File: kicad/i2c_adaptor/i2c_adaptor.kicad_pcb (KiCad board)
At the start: 2 copper layers, 15 parts, among them J1 Conn_01x02, J2 Conn_01x05, J4 Conn_01x14, J5 Conn_01x02, J6 Conn_01x14, Q1 Fairchild BS170, SW1 SW_SPDT, U1 pic16f1825

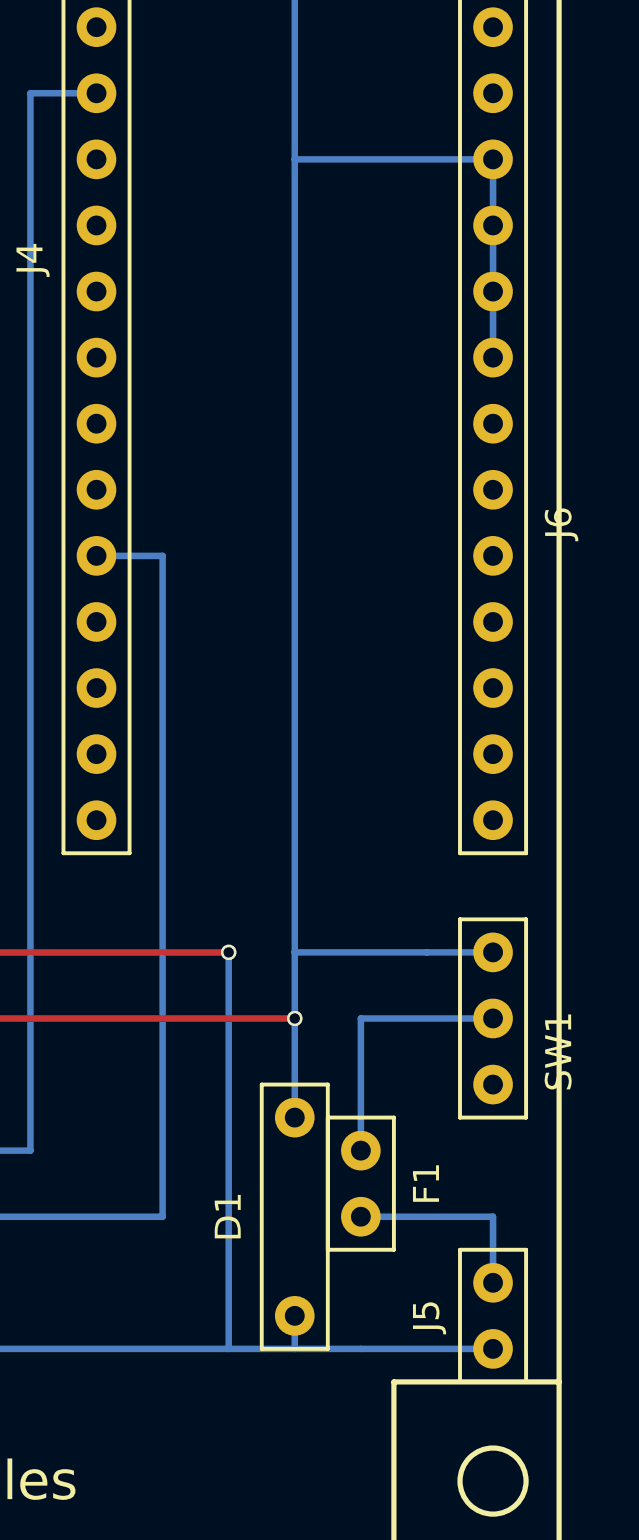
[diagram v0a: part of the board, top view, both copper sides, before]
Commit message: update
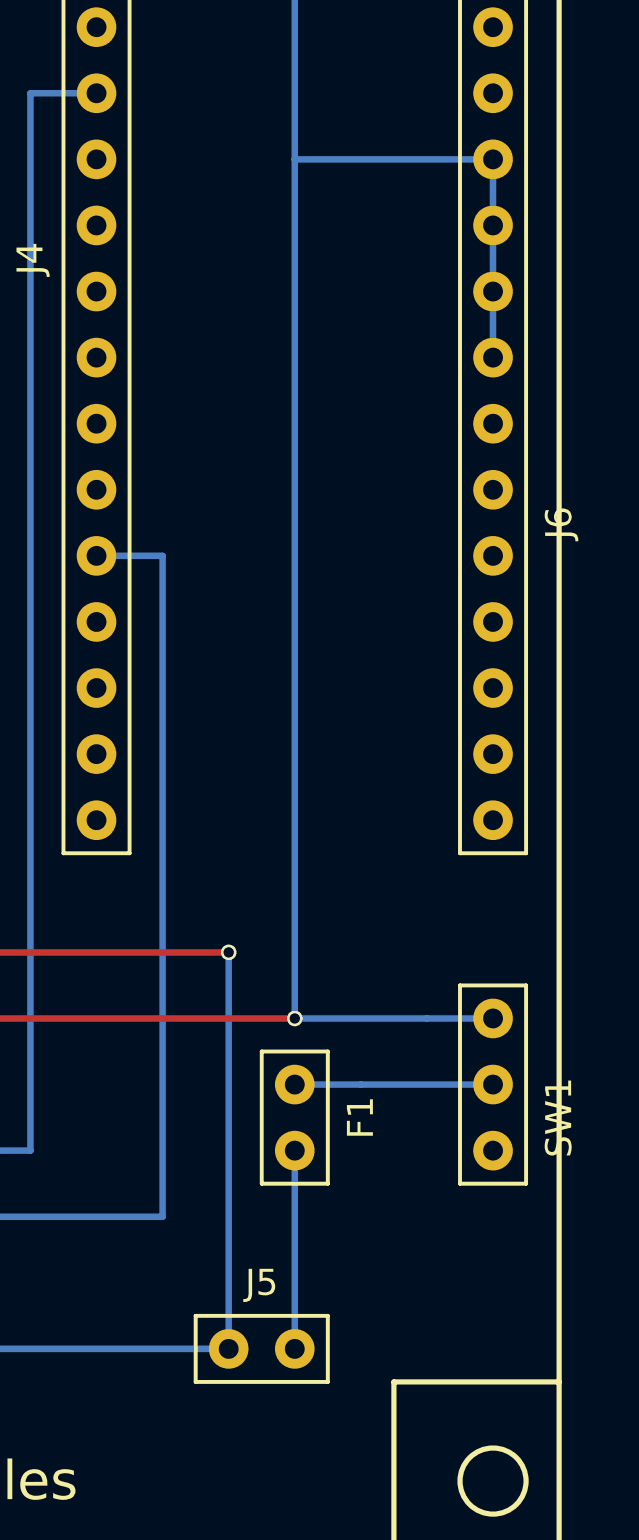
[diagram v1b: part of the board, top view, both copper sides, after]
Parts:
- removed D1: 1A, pic16f1:diode
- moved J5 8.98 mm to (196.8, 135.9), turned to 180 degrees
- moved F1 3.59 mm to (198.1, 127.0)
- moved SW1 2.54 mm to (205.7, 125.7)
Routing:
- net GND: track 90.2 -> 78.7 mm
- net +3V3: track 174.0 -> 170.2 mm
- net Net-(F1-Pad2): track 10.2 -> 7.62 mm
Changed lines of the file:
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@@
 (kicad_pcb (version 4) (host pcbnew 4.0.7)
   (general
-    (links 32)
+    (links 30)
     (no_connects 0)
     (area 0 0 0 0)
     (thickness 1.6)
     (drawings 19)
-    (tracks 76)
+    (tracks 70)
     (zones 0)
-    (modules 15)
+    (modules 14)
     (nets 40)
   )
@@
   )
   (module pic16f1:Capacitor (layer F.Cu)
-    (at 200.66 129.54 90)
+    (at 198.12 127 90)
     (fp_text reference F1 (at 0 2.54 90) (layer F.SilkS)
       (effects (font (size 1 1) (thickness 0.15)))
@@
   )
   (module "mcu:Pin Header 2P" (layer F.Cu)
-    (at 205.74 134.62 270)
-    (fp_text reference J5 (at 0 2.54 270) (layer F.SilkS)
-      (effects (font (size 1 1) (thickness 0.15)))
-    )
-    (fp_text value Conn_01x02 (at 0 -2.54 270) (layer F.Fab)
+    (at 196.85 135.89 180)
+    (fp_text reference J5 (at 0 2.54 180) (layer F.SilkS)
+      (effects (font (size 1 1) (thickness 0.15)))
+    )
+    (fp_text value Conn_01x02 (at 0 -2.54 180) (layer F.Fab)
       (effects (font (size 1 1) (thickness 0.15)))
     )
@@
     (fp_line (start 2.54 1.27) (end 2.54 -1.27) (layer F.SilkS) (width 0.15))
     (fp_line (start 2.54 -1.27) (end -2.54 -1.27) (layer F.SilkS) (width 0.15))
-    (pad 1 thru_hole circle (at -1.27 0 270) (size 1.524 1.524) (drill 0.762) (layers *.Cu *.Mask)
+    (pad 1 thru_hole circle (at -1.27 0 180) (size 1.524 1.524) (drill 0.762) (layers *.Cu *.Mask)
       (net 3 "Net-(F1-Pad1)"))
-    (pad 2 thru_hole circle (at 1.27 0 270) (size 1.524 1.524) (drill 0.762) (layers *.Cu *.Mask)
+    (pad 2 thru_hole circle (at 1.27 0 180) (size 1.524 1.524) (drill 0.762) (layers *.Cu *.Mask)
       (net 2 GND))
   )
@@
   )
   (module mcu:Slide_switch (layer F.Cu)
-    (at 205.74 123.19 90)
+    (at 205.74 125.73 90)
     (fp_text reference SW1 (at -1.27 2.54 90) (layer F.SilkS)
       (effects (font (size 1 1) (thickness 0.15)))
@@
       (net 39 "Net-(J1-Pad2)"))
   )
-  (module pic16f1:diode (layer F.Cu)
-    (at 198.12 130.81 270)
-    (fp_text reference D1 (at 0 2.54 270) (layer F.SilkS)
-      (effects (font (size 1 1) (thickness 0.15)))
-    )
-    (fp_text value 1A (at 0 -2.54 270) (layer F.Fab)
-      (effects (font (size 1 1) (thickness 0.15)))
-    )
-    (fp_line (start -5.08 -1.27) (end -5.08 1.27) (layer F.SilkS) (width 0.15))
-    (fp_line (start -5.08 1.27) (end 5.08 1.27) (layer F.SilkS) (width 0.15))
-    (fp_line (start 5.08 1.27) (end 5.08 -1.27) (layer F.SilkS) (width 0.15))
-    (fp_line (start 5.08 -1.27) (end -5.08 -1.27) (layer F.SilkS) (width 0.15))
-    (pad 1 thru_hole circle (at -3.81 0 270) (size 1.524 1.524) (drill 0.762) (layers *.Cu *.Mask)
-      (net 1 +3V3))
-    (pad 2 thru_hole circle (at 3.81 0 270) (size 1.524 1.524) (drill 0.762) (layers *.Cu *.Mask)
-      (net 2 GND))
-  )
   (gr_line (start 208.28 143.51) (end 162.56 143.51) (angle 90) (layer F.SilkS) (width 0.2))
   (gr_line (start 208.28 72.39) (end 208.28 143.51) (angle 90) (layer F.SilkS) (width 0.2))
@@
   (gr_line (start 208.28 72.39) (end 162.56 72.39) (angle 90) (layer F.SilkS) (width 0.2))
   (segment (start 185.42 99.06) (end 185.42 99.06) (width 0.25) (layer B.Cu) (net 0))
-  (segment (start 198.12 127) (end 198.12 123.19) (width 0.25) (layer B.Cu) (net 1) (status 400000))
   (segment (start 167.64 130.81) (end 167.64 128.27) (width 0.25) (layer B.Cu) (net 1))
   (segment (start 185.42 123.19) (end 198.12 123.19) (width 0.25) (layer F.Cu) (net 1))
   (segment (start 165.1 123.19) (end 185.42 123.19) (width 0.25) (layer B.Cu) (net 1))
-  (segment (start 198.12 123.19) (end 198.12 120.65) (width 0.25) (layer B.Cu) (net 1))
+  (segment (start 198.12 123.19) (end 198.12 123.19) (width 0.25) (layer B.Cu) (net 1))
   (via (at 198.12 123.19) (size 0.6) (drill 0.4) (layers F.Cu B.Cu) (net 1))
   (via (at 185.42 123.19) (size 0.6) (drill 0.4) (layers F.Cu B.Cu) (net 1))
   (segment (start 205.74 90.17) (end 198.12 90.17) (width 0.25) (layer B.Cu) (net 1))
   (segment (start 205.74 82.55) (end 198.12 82.55) (width 0.25) (layer B.Cu) (net 1))
-  (segment (start 198.12 120.65) (end 198.12 90.17) (width 0.25) (layer B.Cu) (net 1))
+  (segment (start 198.12 123.19) (end 198.12 90.17) (width 0.25) (layer B.Cu) (net 1))
   (segment (start 198.12 90.17) (end 198.12 82.55) (width 0.25) (layer B.Cu) (net 1))
   (segment (start 198.12 82.55) (end 198.12 80.01) (width 0.25) (layer B.Cu) (net 1))
@@
   (segment (start 205.74 92.71) (end 205.74 95.25) (width 0.25) (layer B.Cu) (net 1))
   (segment (start 205.74 95.25) (end 205.74 97.79) (width 0.25) (layer B.Cu) (net 1))
-  (segment (start 203.2 120.65) (end 198.12 120.65) (width 0.25) (layer B.Cu) (net 1))
-  (segment (start 203.2 120.65) (end 205.74 120.65) (width 0.25) (layer B.Cu) (net 1) (status 20))
+  (segment (start 203.2 123.19) (end 198.12 123.19) (width 0.25) (layer B.Cu) (net 1))
+  (segment (start 203.2 123.19) (end 205.74 123.19) (width 0.25) (layer B.Cu) (net 1) (status 20))
   (segment (start 165.1 123.19) (end 165.1 125.73) (width 0.25) (layer B.Cu) (net 1))
   (segment (start 165.1 125.73) (end 167.64 125.73) (width 0.25) (layer B.Cu) (net 1))
   (segment (start 167.64 102.87) (end 167.64 100.33) (width 0.25) (layer B.Cu) (net 1))
   (segment (start 167.64 128.27) (end 167.64 125.73) (width 0.25) (layer B.Cu) (net 1) (status 10))
-  (segment (start 198.12 134.62) (end 198.12 135.89) (width 0.25) (layer B.Cu) (net 2) (status 400000))
   (segment (start 177.8 135.89) (end 195.58 135.89) (width 0.25) (layer B.Cu) (net 2))
   (segment (start 185.42 120.65) (end 195.58 120.65) (width 0.25) (layer F.Cu) (net 2))
   (segment (start 185.42 120.65) (end 185.42 110.49) (width 0.25) (layer B.Cu) (net 2) (status 20))
-  (segment (start 200.66 135.89) (end 198.12 135.89) (width 0.25) (layer B.Cu) (net 2))
-  (segment (start 198.12 135.89) (end 195.58 135.89) (width 0.25) (layer B.Cu) (net 2))
   (segment (start 195.58 135.89) (end 195.58 120.65) (width 0.25) (layer B.Cu) (net 2))
-  (segment (start 200.66 135.89) (end 205.74 135.89) (width 0.25) (layer B.Cu) (net 2) (status 20))
   (segment (start 165.1 120.65) (end 185.42 120.65) (width 0.25) (layer B.Cu) (net 2))
   (via (at 185.42 120.65) (size 0.6) (drill 0.4) (layers F.Cu B.Cu) (net 2))
@@
   (segment (start 167.64 118.11) (end 165.1 118.11) (width 0.25) (layer B.Cu) (net 2))
   (segment (start 165.1 118.11) (end 165.1 120.65) (width 0.25) (layer B.Cu) (net 2))
-  (segment (start 200.66 130.81) (end 205.74 130.81) (width 0.25) (layer B.Cu) (net 3))
-  (segment (start 205.74 130.81) (end 205.74 133.35) (width 0.25) (layer B.Cu) (net 3) (status 20))
-  (segment (start 205.74 123.19) (end 200.66 123.19) (width 0.25) (layer B.Cu) (net 4))
-  (segment (start 200.66 123.19) (end 200.66 128.27) (width 0.25) (layer B.Cu) (net 4))
+  (segment (start 198.12 128.27) (end 198.12 135.89) (width 0.25) (layer B.Cu) (net 3) (status C00000))
+  (segment (start 205.74 125.73) (end 200.66 125.73) (width 0.25) (layer B.Cu) (net 4) (status 10))
+  (segment (start 200.66 125.73) (end 198.12 125.73) (width 0.25) (layer B.Cu) (net 4) (status 20))
   (segment (start 175.26 100.33) (end 175.26 102.87) (width 0.25) (layer B.Cu) (net 6) (status 10))
   (segment (start 175.26 102.87) (end 175.26 115.57) (width 0.25) (layer B.Cu) (net 6))
